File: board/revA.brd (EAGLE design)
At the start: 40 x 50 mm, 28 parts, among them IC1 LM2931, U1 LDK120DM33R

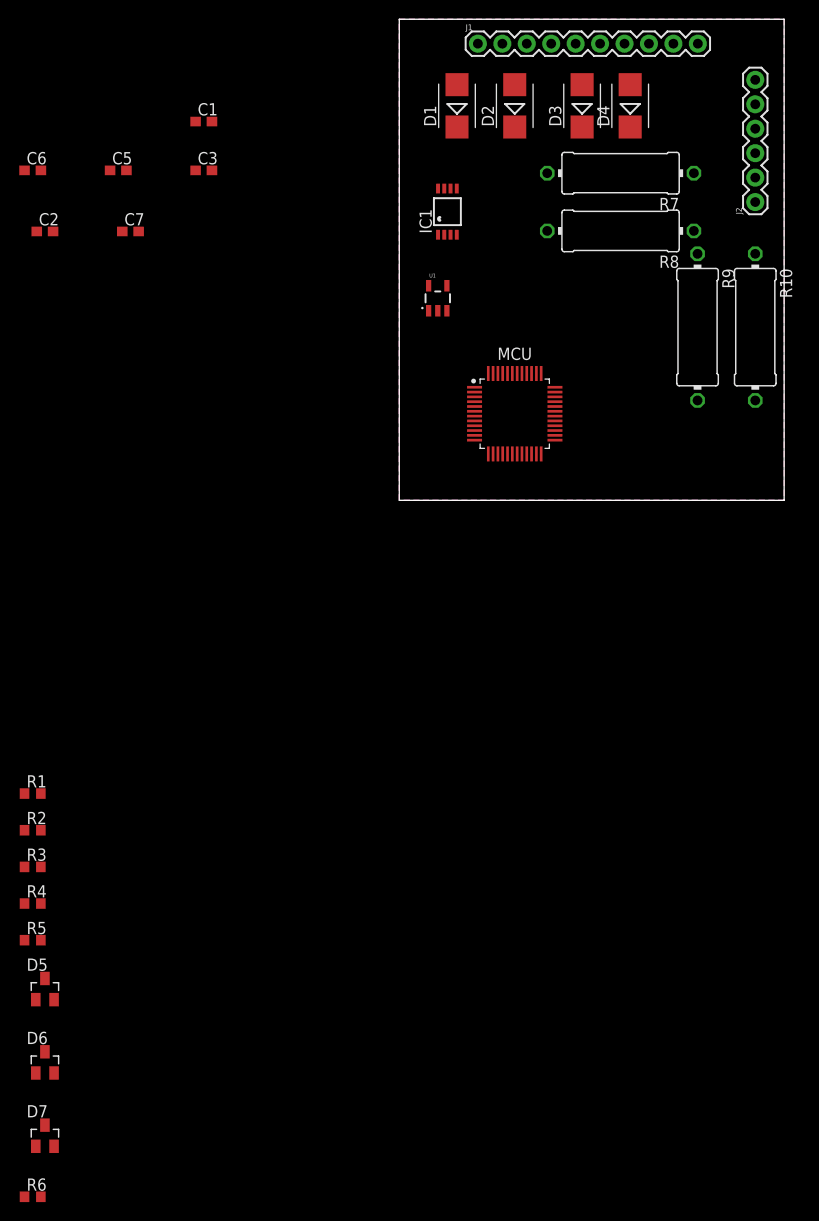
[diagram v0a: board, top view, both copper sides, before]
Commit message: Updating values
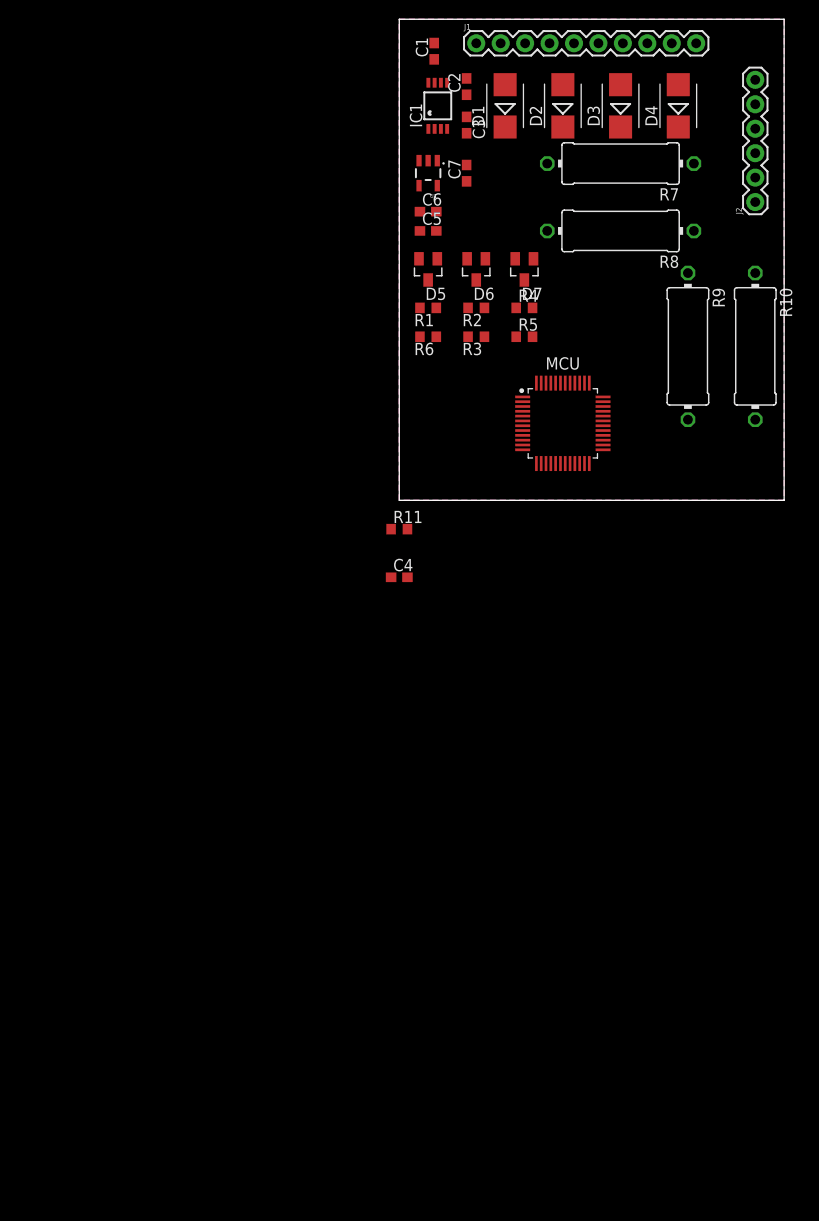
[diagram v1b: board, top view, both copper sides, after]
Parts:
- added C4: 1uF 5v, rcl:C0603
- added R11: 10k, rcl:R0603
- D1, D2, D3, D4: value (none) -> 80V
- R10, R7, R8, R9: value (none) -> 470R
- moved D7 102.9 mm to (13.0, 24.0), turned to 180 degrees
- moved R6 98.4 mm to (3.00, 17.0), turned to 180 degrees
- moved D6 93.8 mm to (8.00, 24.0), turned to 180 degrees
- moved D5 84.7 mm to (3.00, 24.0), turned to 180 degrees
- moved R5 80.9 mm to (13.0, 17.0)
- moved R4 80.3 mm to (13.0, 20.0)
- moved R3 71.8 mm to (8.00, 17.0), turned to 180 degrees
- moved R2 71.2 mm to (8.00, 20.0), turned to 180 degrees
- moved R1 65.1 mm to (3.00, 20.0), turned to 180 degrees
- moved C2 46.3 mm to (7.00, 43.0), turned to 90 degrees
- moved C6 41.3 mm to (3.00, 30.0)
- moved C7 35.5 mm to (7.00, 34.0), turned to 90 degrees
- moved C5 32.8 mm to (3.00, 28.0)
- moved C3 27.7 mm to (7.00, 39.0), turned to 270 degrees
- moved C1 25.0 mm to (3.63, 46.7), turned to 90 degrees
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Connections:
- removed net VBAT: MCU.1
- removed net VDDA: MCU.9
- removed net VDD_1: MCU.24
- removed net VDD_2: MCU.36
- removed net VDD_3: MCU.48
- removed net VSSA: MCU.8
- removed net VSS_1: MCU.23
- removed net VSS_2: MCU.35
- removed net VSS_3: MCU.47
- new net N$1: C4.1, R11.2
- new net NRST: C4.2, MCU.7
- net +3V3: now also MCU.1, MCU.24, MCU.36, MCU.44, MCU.48, MCU.9, R11.1
- net GND: now also MCU.23, MCU.35, MCU.47, MCU.8
